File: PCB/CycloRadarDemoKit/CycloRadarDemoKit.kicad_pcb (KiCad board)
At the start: 2 copper layers, 66.6 x 44.8 mm, 8 parts, among them Q301 L8050QLT1G, Q302 L8050QLT1G, U101 ESP32-WROVER-E, U201 IP101GRI, U301 CP2102N-Axx-xQFN28

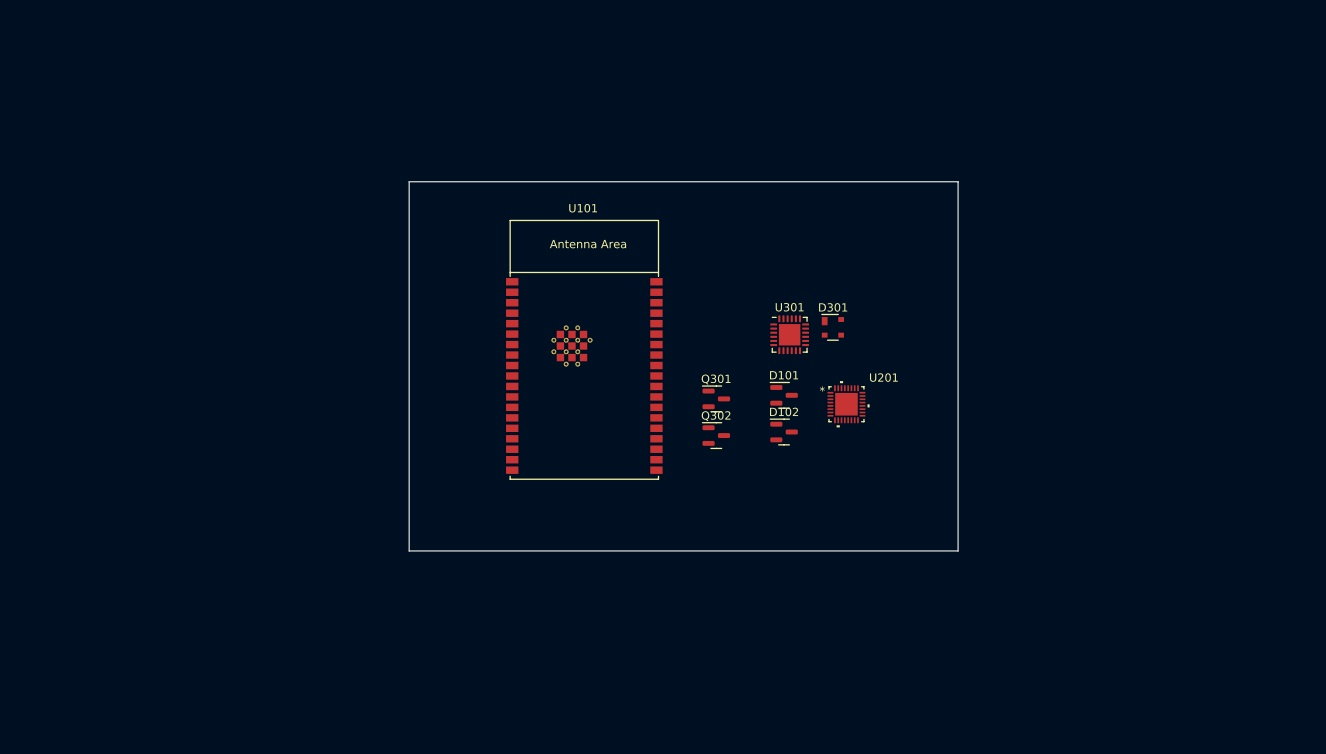
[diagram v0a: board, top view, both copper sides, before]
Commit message: PCB power manag. WIP
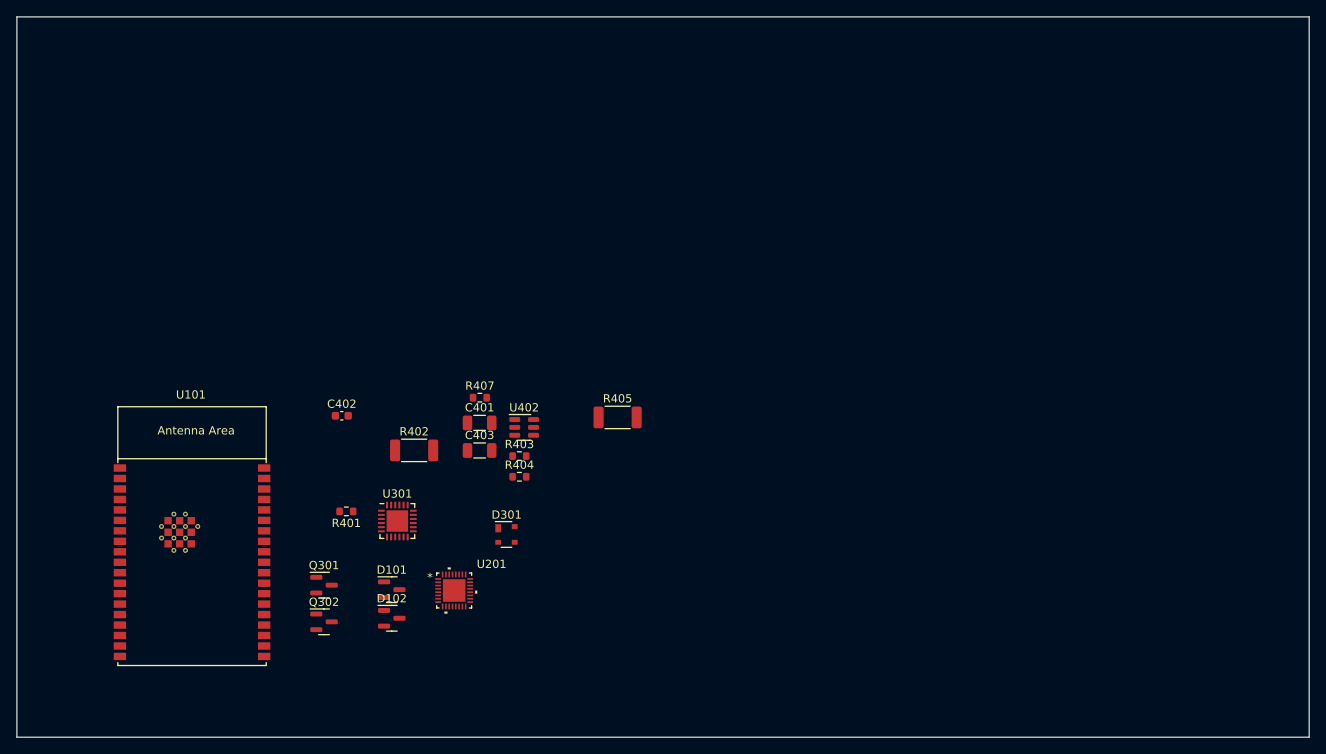
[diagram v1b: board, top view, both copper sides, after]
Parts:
- added C401: 10uF/25V(10%), Capacitor_SMD:C_1206_3216Metric, F.Cu at (125.5, 102.1)
- added C402: 10nF/50V(10%), Capacitor_SMD:C_0603_1608Metric, F.Cu at (108.8, 101.2)
- added C403: 22uF/16V(20%), Capacitor_SMD:C_1206_3216Metric, F.Cu at (125.5, 105.4)
- added R401: 0R, Resistor_SMD:R_0603_1608Metric, F.Cu at (109.4, 112.8)
- added R402: 0.2R(1%), Resistor_SMD:R_2010_5025Metric, F.Cu at (117.6, 105.4)
- added R403: 51K(1%), Resistor_SMD:R_0603_1608Metric, F.Cu at (130.4, 106.1)
- added R404: 3.6K(1%), Resistor_SMD:R_0603_1608Metric, F.Cu at (130.4, 108.6)
- added R405: R_Shunt, Resistor_SMD:R_2010_5025Metric, F.Cu at (142.3, 101.4)
- added R407: 0R, Resistor_SMD:R_0603_1608Metric, F.Cu at (125.6, 99.0)
- added U402: RT8259, Package_TO_SOT_SMD:TSOT-23-6, F.Cu at (130.9, 102.6)
- moved D101 53.1 mm to (114.9, 122.3)
- moved U201 52.7 mm to (122.5, 122.4)
- moved D102 52.7 mm to (114.9, 125.8)
- moved Q301 52.7 mm to (106.7, 121.8)
- moved Q302 52.7 mm to (106.7, 126.2)
- moved U101 52.7 mm to (90.7, 115.8)
- moved U301 52.7 mm to (115.6, 114.0)
- moved D301 46.9 mm to (128.8, 115.6)
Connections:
- U101 pad 1: Net-(U101-GND-Pad1) -> GND
- U101 pad 10: unconnected-(U101-DAC_1/ADC2_CH8/GPIO25-Pad10) -> /MAC_RXD0
- U101 pad 11: unconnected-(U101-DAC_2/ADC2_CH9/GPIO26-Pad11) -> /MAC_RXD1
- U101 pad 12: unconnected-(U101-ADC2_CH7/GPIO27-Pad12) -> /MAC_CRS_DV
- U101 pad 13: unconnected-(U101-MTMS/GPIO14/ADC2_CH6-Pad13) -> /TMS
- U101 pad 14: unconnected-(U101-MTDI/GPIO12/ADC2_CH5-Pad14) -> /TDI
- U101 pad 15: Net-(U101-GND-Pad1) -> GND
- U101 pad 16: unconnected-(U101-MTCK/GPIO13/ADC2_CH4-Pad16) -> /TCK
- U101 pad 2: unconnected-(U101-3V3-Pad2) -> +3V3
- U101 pad 23: unconnected-(U101-MTDO/GPIO15/ADC2_CH3-Pad23) -> /TDO
- U101 pad 24: unconnected-(U101-ADC2_CH2/GPIO2-Pad24) -> /GPIO2
- U101 pad 25: unconnected-(U101-GPIO0/BOOT/ADC2_CH1-Pad25) -> /MAC_CLK
- U101 pad 29: unconnected-(U101-GPIO5-Pad29) -> /PHY_RST
- U101 pad 3: unconnected-(U101-EN/CHIP_PU-Pad3) -> /EN
- U101 pad 30: unconnected-(U101-GPIO18-Pad30) -> /MAC_MDIO
- U101 pad 31: unconnected-(U101-GPIO19-Pad31) -> /MAC_TXD(0)
- U101 pad 33: unconnected-(U101-GPIO21-Pad33) -> /MAC_TX_EN
- U101 pad 34: unconnected-(U101-U0RXD/GPIO3-Pad34) -> /U0RXD
- U101 pad 35: unconnected-(U101-U0TXD/GPIO1-Pad35) -> /U0TXD
- U101 pad 36: unconnected-(U101-GPIO22-Pad36) -> /MAC_TXD(1)
- U101 pad 37: unconnected-(U101-GPIO23-Pad37) -> /MAC_MDC
- U101 pad 38: Net-(U101-GND-Pad1) -> GND
- U101 pad 39: unconnected-(U101-GND_THERMAL-Pad39) -> GND
- U201 pad 10: /IO0 -> /MAC_CLK
- U201 pad 14: /IO0 -> /MAC_CLK
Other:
- board size 66.6 x 44.8 mm -> 156.8 x 87.4 mm
